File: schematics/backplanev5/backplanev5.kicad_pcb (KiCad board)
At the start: 2 copper layers, 150 x 102.7 mm, 28 parts, among them J12 Conn_01x02, J13 Conn_01x02, J14 Conn_01x02

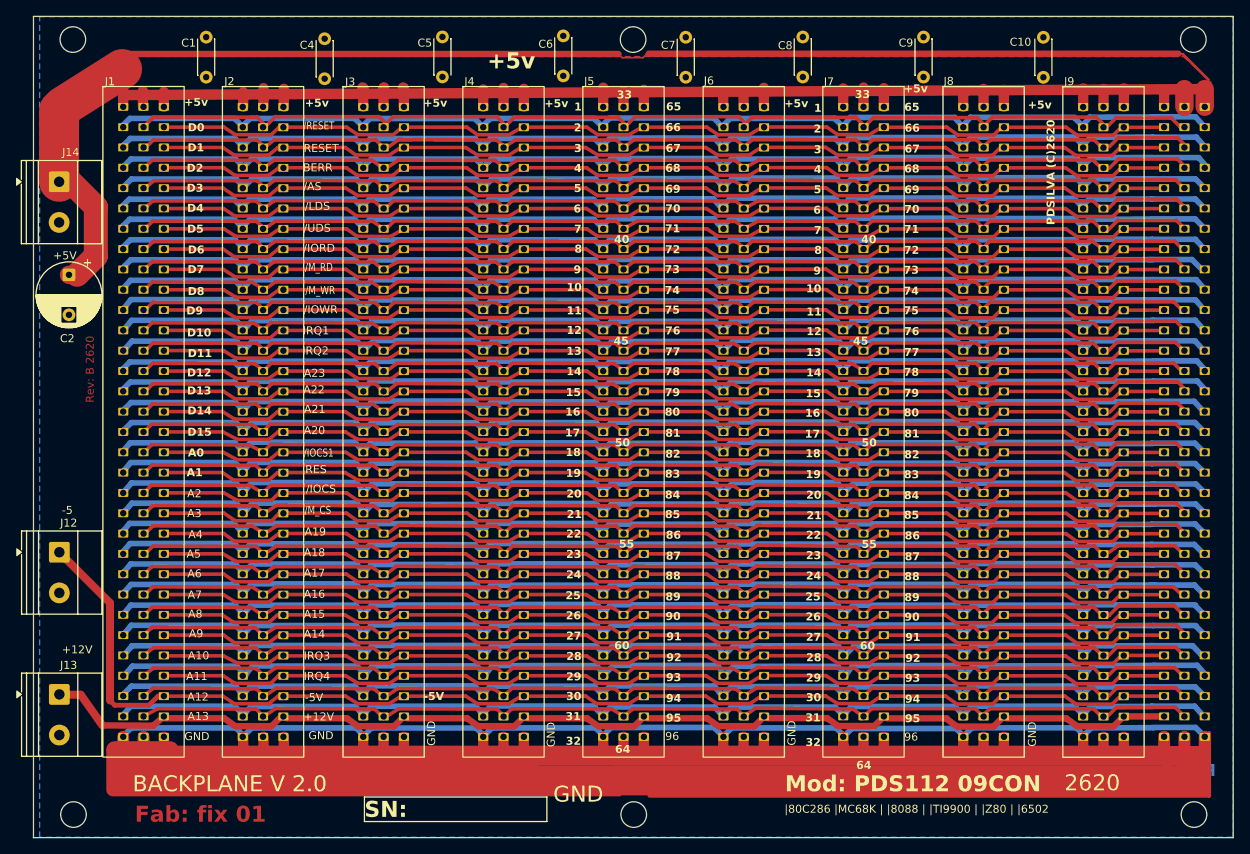
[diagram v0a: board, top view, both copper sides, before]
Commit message: Enviado arquivo Gerber_fab_2620_02.zip para TEC-CI
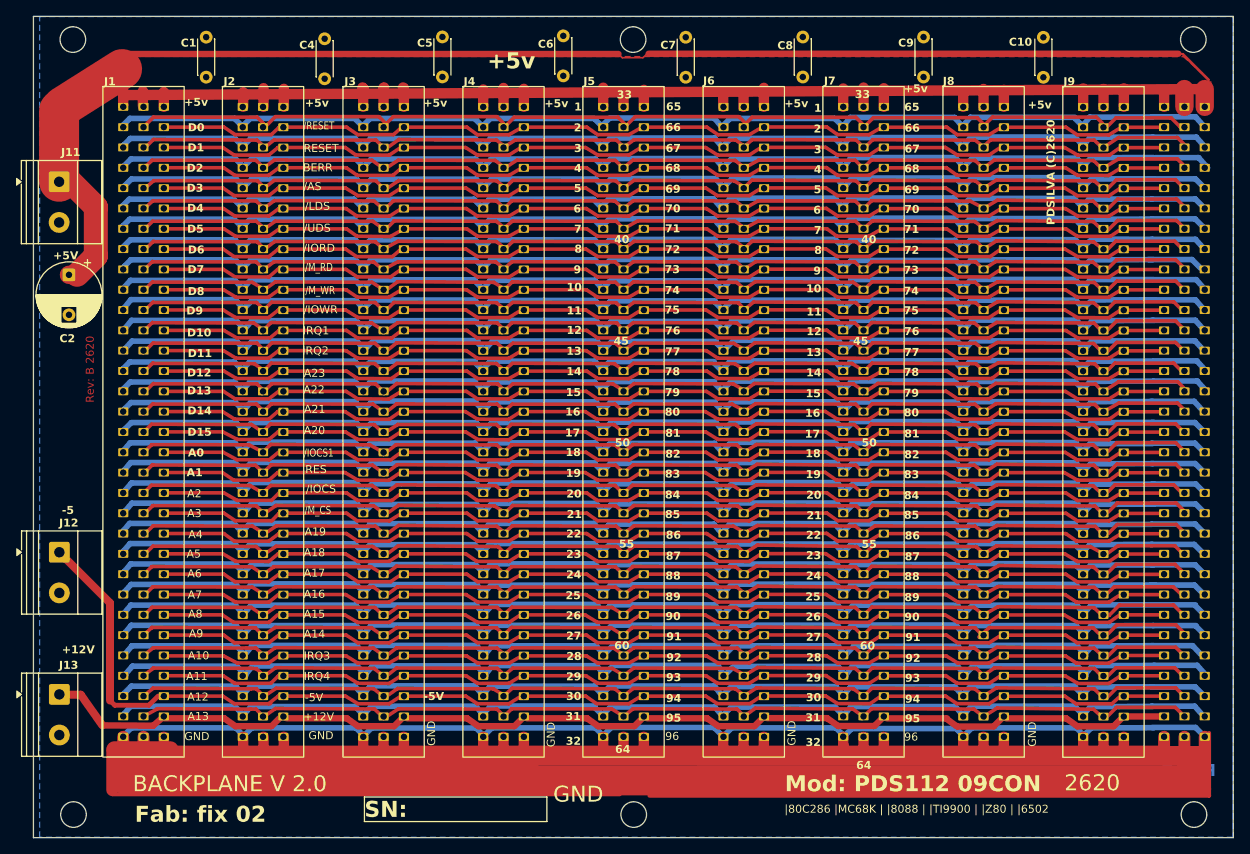
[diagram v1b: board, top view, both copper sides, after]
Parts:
- renumbered J14 to J11
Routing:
- net /backplane/R23: track 135.9 -> 134.9 mm
- net /backplane/R29: track 135.6 -> 134.7 mm
- net /backplane/R19: track 135.8 -> 134.9 mm
- net /backplane/R7: track 136.7 -> 135.8 mm
- net /backplane/R5: track 136.5 -> 135.7 mm
- net /backplane/R6: track 135.7 -> 134.9 mm
- net /backplane/R12: track 136.3 -> 135.5 mm
- net /backplane/R17: track 135.6 -> 134.9 mm
- net /backplane/R25: track 136.3 -> 135.5 mm
- net /backplane/R16: track 135.7 -> 134.9 mm
- net /backplane/R30: track 136.2 -> 135.4 mm
- net /backplane/R11: track 136.4 -> 135.6 mm
- net /backplane/R22: track 136.0 -> 135.2 mm
- net /backplane/R8: track 135.7 -> 134.9 mm
- net /backplane/R27: track 135.7 -> 135.0 mm
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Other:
- board text added: "Fab: fix 02"
- board text removed: "Fab: fix 01"
